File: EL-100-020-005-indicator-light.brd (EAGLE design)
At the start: 20 x 39.8 mm, 13 parts, among them X1 140-08-FLACHBAND1.27

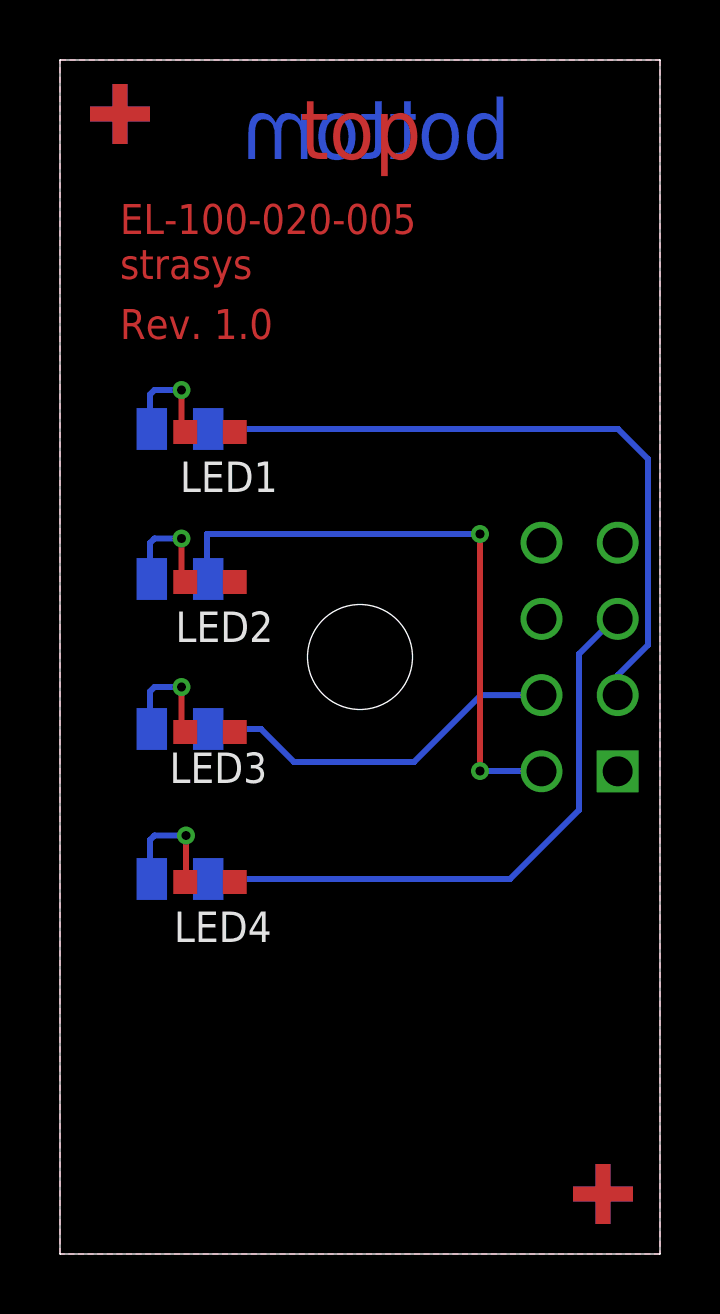
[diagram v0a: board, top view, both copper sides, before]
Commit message: DIN-Rail-production
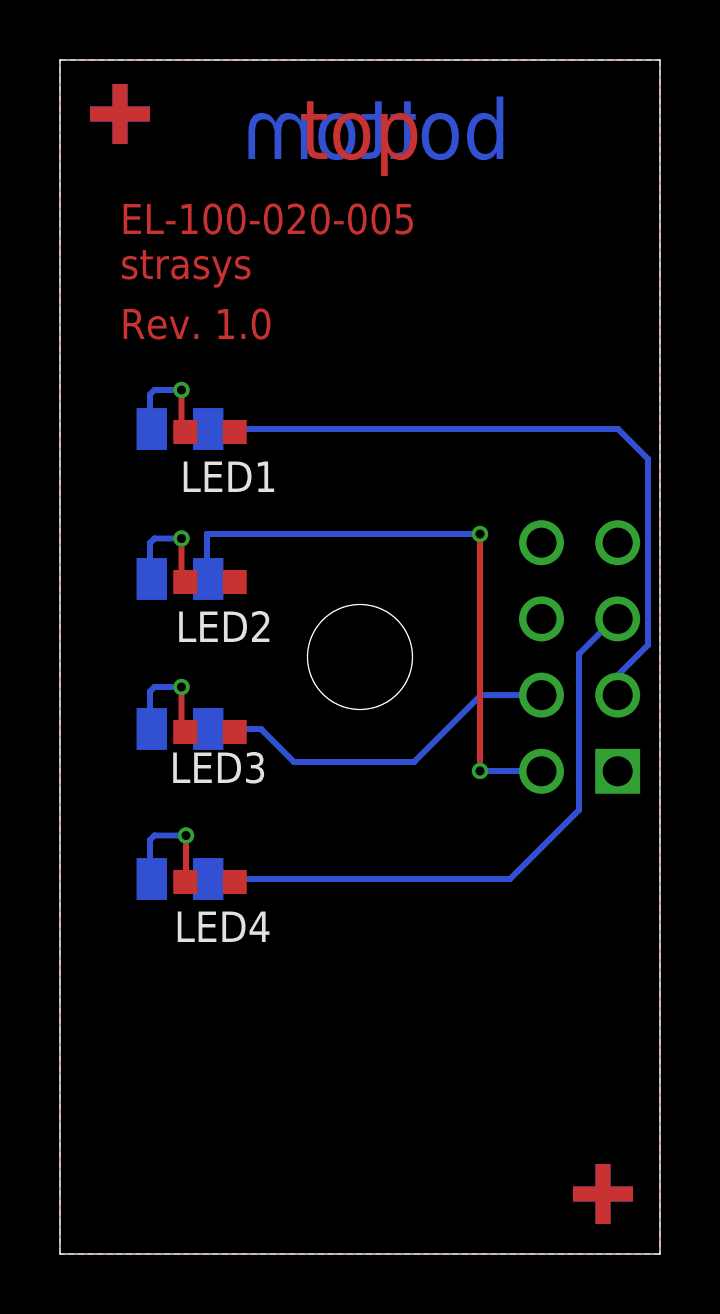
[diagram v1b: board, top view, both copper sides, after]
